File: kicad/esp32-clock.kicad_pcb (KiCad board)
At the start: 2 copper layers, 112.5 x 64 mm, 34 parts, among them J1 Battery Connector, P1 USB_C_Plug_USB2.0, SW1 RESET, SW2 BOOT, U1 ESP-12E, U2 CP2102N-Axx-xQFN20, U3 MCP73831-2-OT, U4 BCM857BS, U5 ME6211C12M5G-N

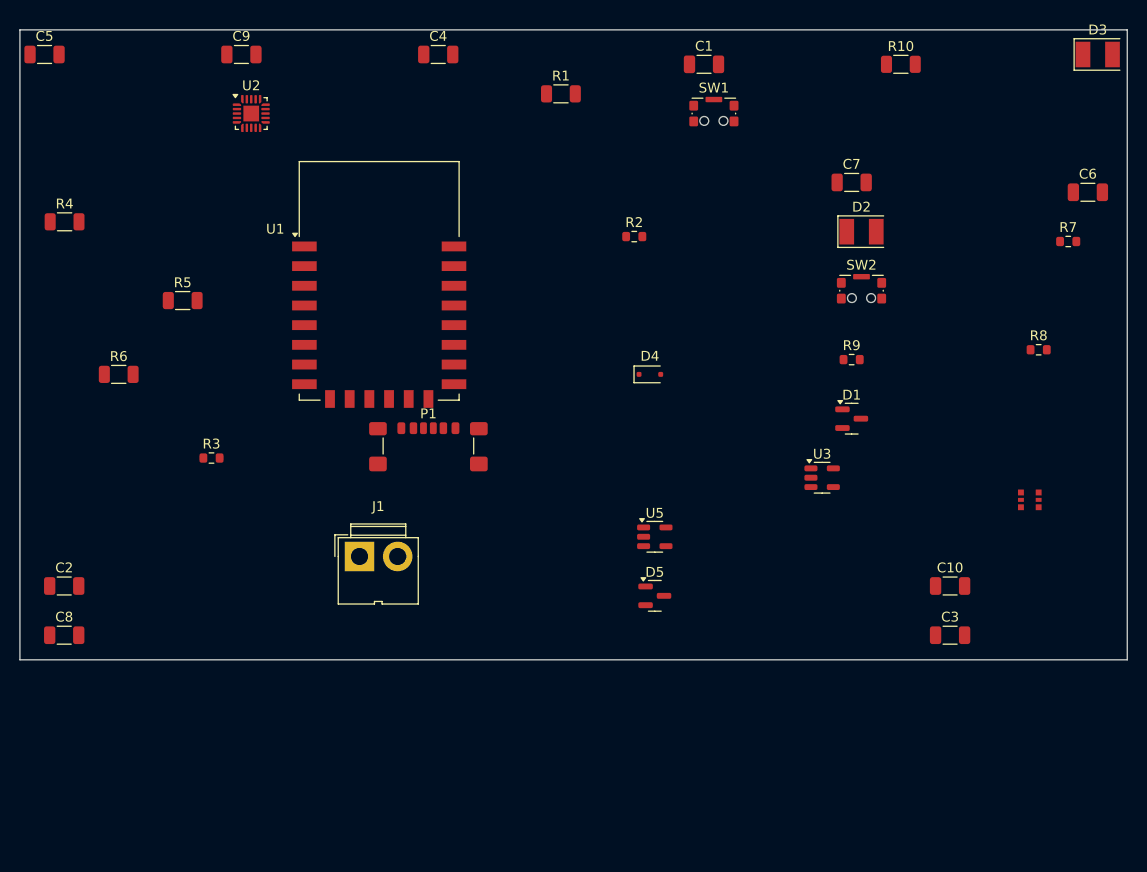
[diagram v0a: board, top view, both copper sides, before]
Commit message: init
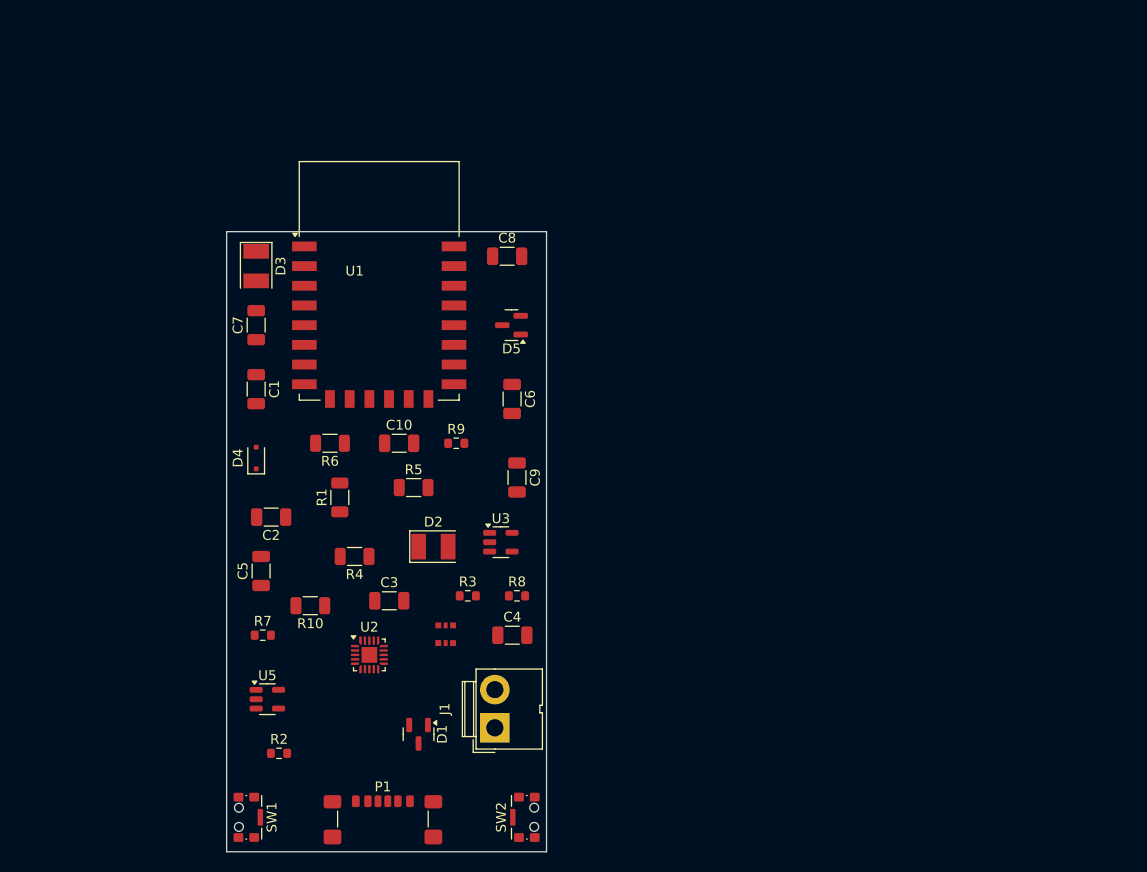
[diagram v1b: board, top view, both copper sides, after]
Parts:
- moved R7 91.1 mm to (86.2, 112.0)
- moved D3 88.2 mm to (85.5, 74.5), turned to -90 degrees
- moved SW1 85.8 mm to (84.5, 130.5), turned to -90 degrees
- moved R10 81.4 mm to (91.0, 109.0), turned to 180 degrees
- moved R2 63.7 mm to (87.8, 124.0)
- moved SW2 63.4 mm to (113.0, 130.5), turned to 90 degrees
- moved C7 62.2 mm to (85.5, 80.5), turned to 90 degrees
- moved C6 62.2 mm to (111.5, 88.0), turned to -90 degrees
- moved U4 60.9 mm to (104.8, 111.9), turned to 90 degrees
- moved C4 59.5 mm to (111.5, 112.0)
- moved C8 59.2 mm to (111.0, 73.5)
- moved R8 58.6 mm to (112.0, 108.0)
- moved C10 57.8 mm to (100.0, 92.5)
- moved C3 57.1 mm to (99.0, 108.5)
- moved C5 56.9 mm to (86.0, 105.5), turned to 90 degrees
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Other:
- board size 112.5 x 64 mm -> 32.5 x 63 mm

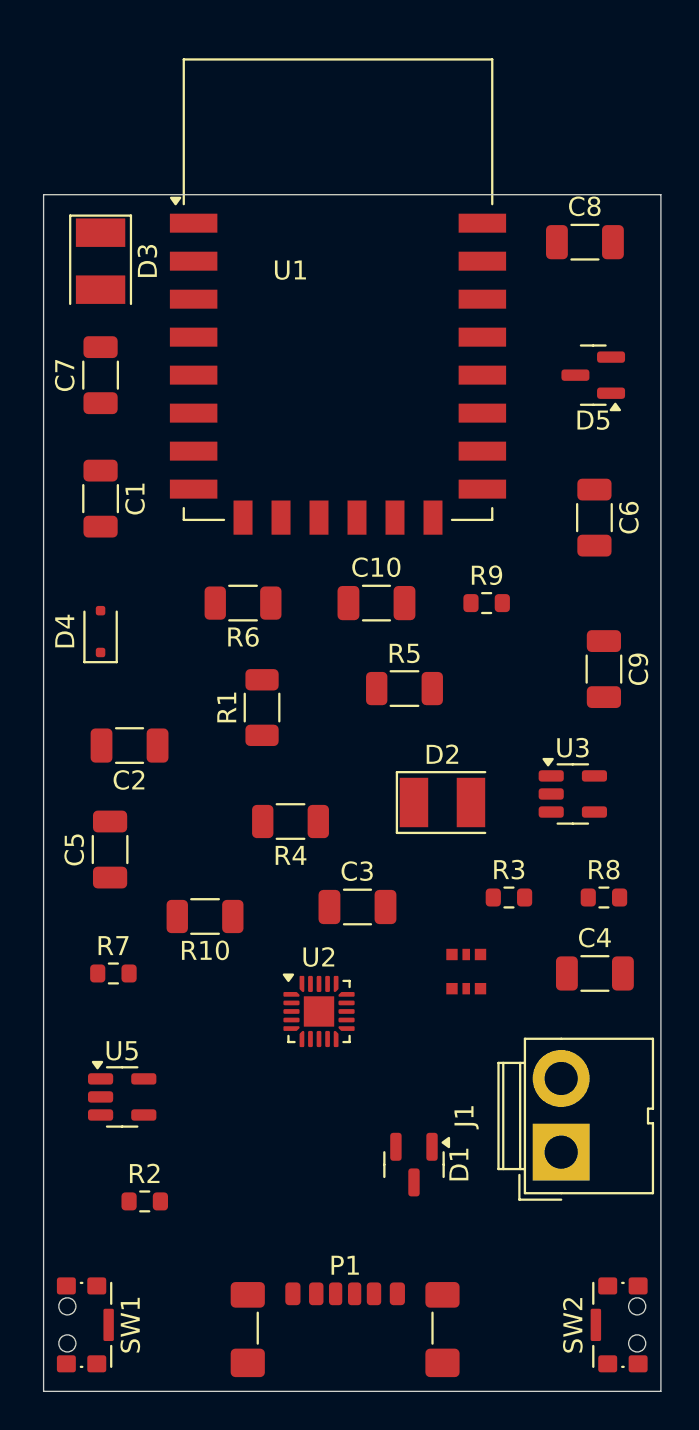
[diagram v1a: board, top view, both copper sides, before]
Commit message: init
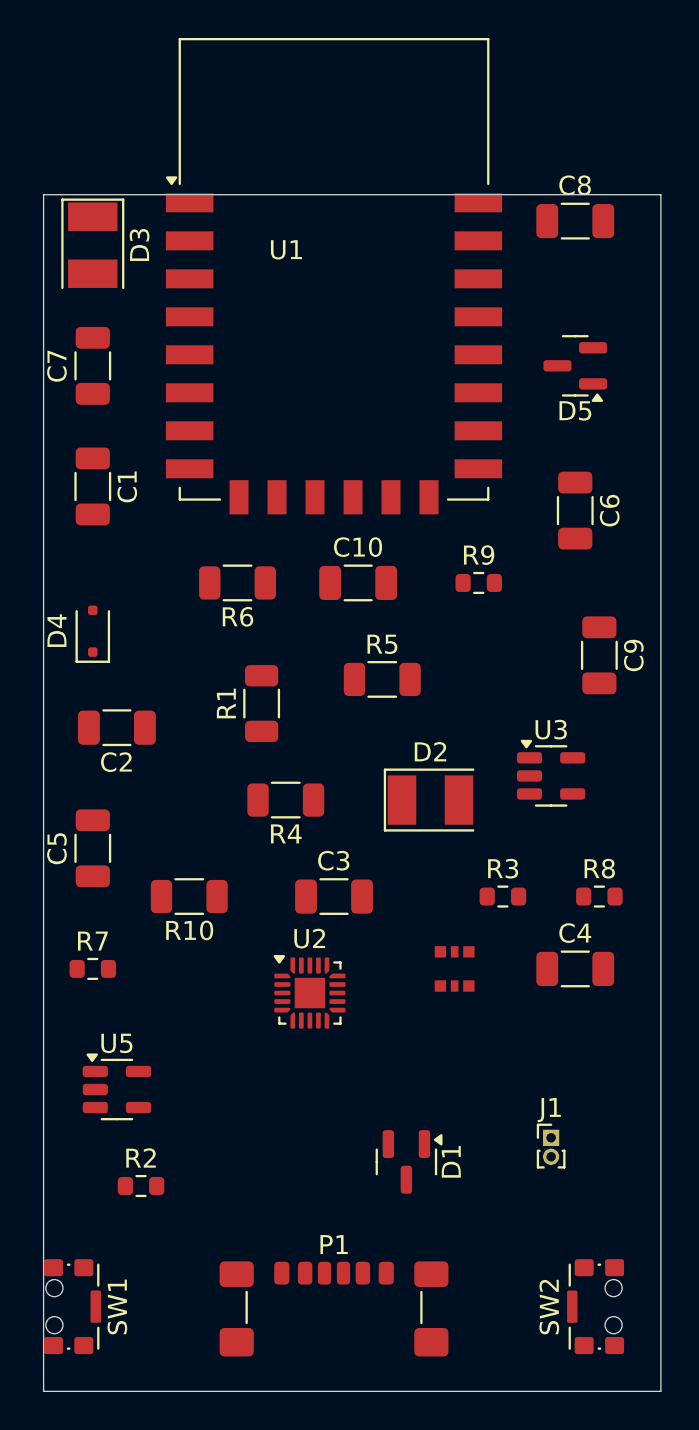
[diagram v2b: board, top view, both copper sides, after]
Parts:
- J1: footprint Connector:JWT_A3963_1x02_P3.96mm_Vertical -> Connector_PinHeader_1.00mm:PinHeader_1x02_P1.00mm_Vertical
- moved SW2 1.57 mm to (111.8, 129.5)
- moved U3 1.49 mm to (109.2, 101.6)
- moved C10 1.43 mm to (99.1, 91.4)
- moved C3 1.35 mm to (97.8, 108.0)
- moved R10 1.34 mm to (90.2, 108.0)
- moved R5 1.26 mm to (100.3, 96.5)
- moved P1 1.23 mm to (97.8, 130.8)
- moved C8 1.22 mm to (110.5, 72.4)
- moved SW1 1.18 mm to (83.8, 129.5)
- moved R4 1.16 mm to (95.2, 102.9)
- moved C2 1.15 mm to (86.4, 99.1)
- moved R9 1.14 mm to (105.4, 91.4)
- moved R7 1.11 mm to (85.1, 111.8)
- moved R6 1.10 mm to (92.7, 91.4)
- moved U1 1.09 mm to (97.8, 74.9)
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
